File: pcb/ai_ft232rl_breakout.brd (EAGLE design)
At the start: 25.4 x 16.3 mm, 14 parts, among them U1 FT232RLSSOP

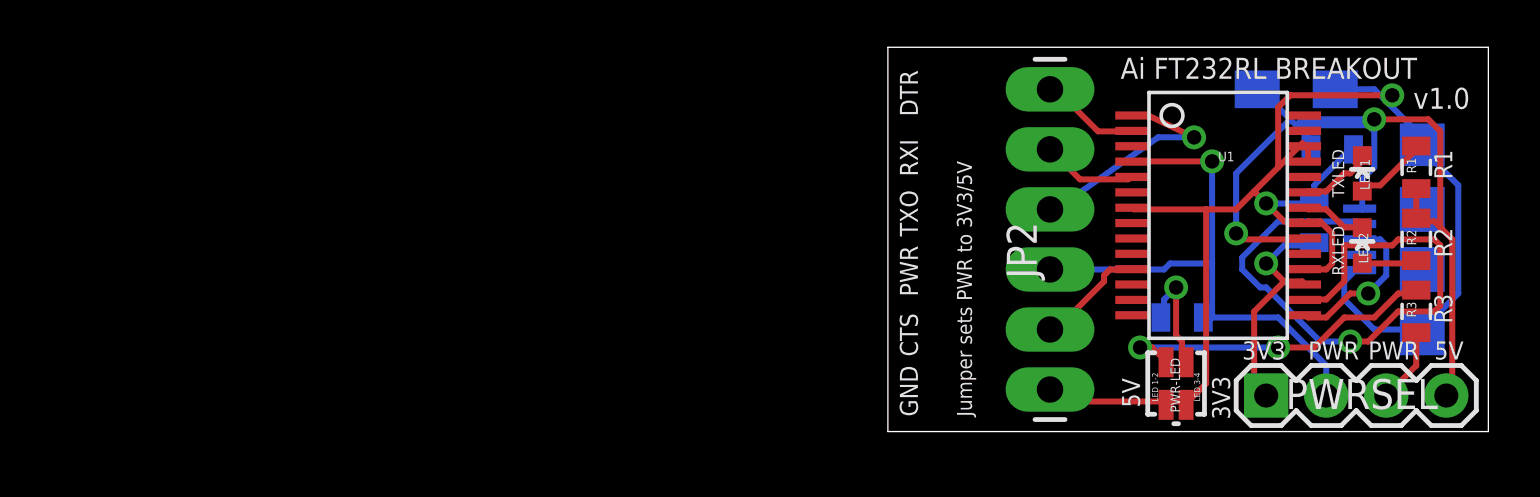
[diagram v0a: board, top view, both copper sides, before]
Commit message: aligned board to origin.
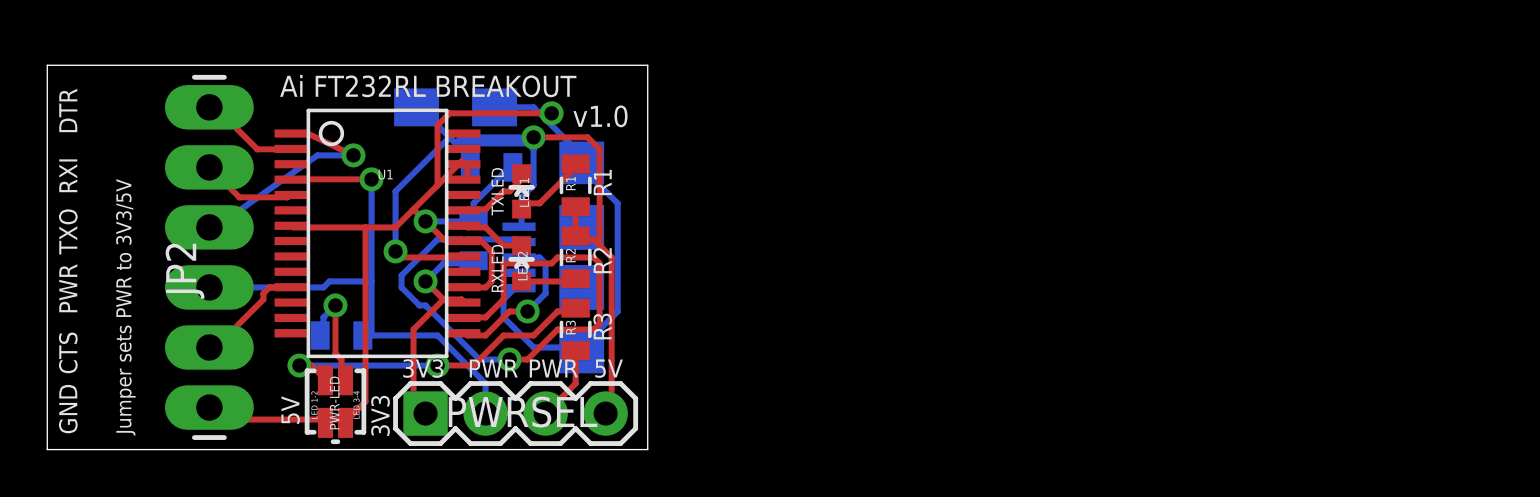
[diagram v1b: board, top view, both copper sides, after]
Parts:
- moved C1 35.6 mm to (18.8, 11.9)
- moved C2 35.6 mm to (18.0, 8.89)
- moved C3 35.6 mm to (17.3, 14.5)
- moved JP2 35.6 mm to (6.86, 1.78)
- moved LED1 35.6 mm to (20.1, 10.9)
- moved LED2 35.6 mm to (20.1, 7.87)
- moved PWR-LED 35.6 mm to (12.2, 2.03)
- moved PWRSEL 35.6 mm to (16.0, 1.52)
- moved R1 35.6 mm to (22.4, 11.2)
- moved R2 35.6 mm to (22.4, 8.13)
- moved R3 35.6 mm to (22.4, 5.08)
- moved R4 35.6 mm to (12.4, 4.83)
- moved U1 35.6 mm to (14.0, 9.14)
- moved USB 35.6 mm to (22.6, 8.13)
